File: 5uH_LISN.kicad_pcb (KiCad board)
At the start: 2 copper layers, 112.4 x 60.5 mm, 74 parts, among them J1 Conn_SMA, J2 Conn_SMA, J3 BANANA_CONN, J4 BANANA_CONN, J5 BANANA_CONN, J6 BANANA_CONN, J7 BANANA_CONN, J8 BANANA_CONN

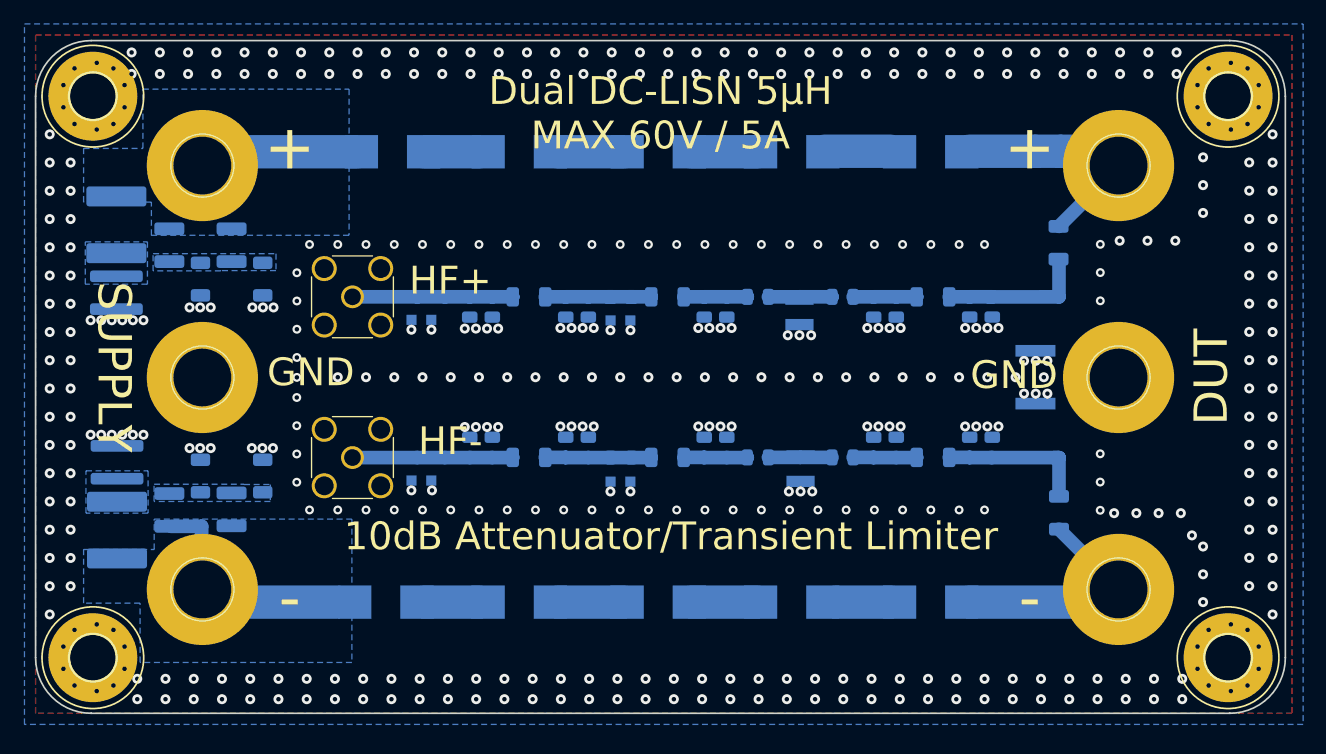
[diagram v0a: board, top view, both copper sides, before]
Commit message: redesign, see readme
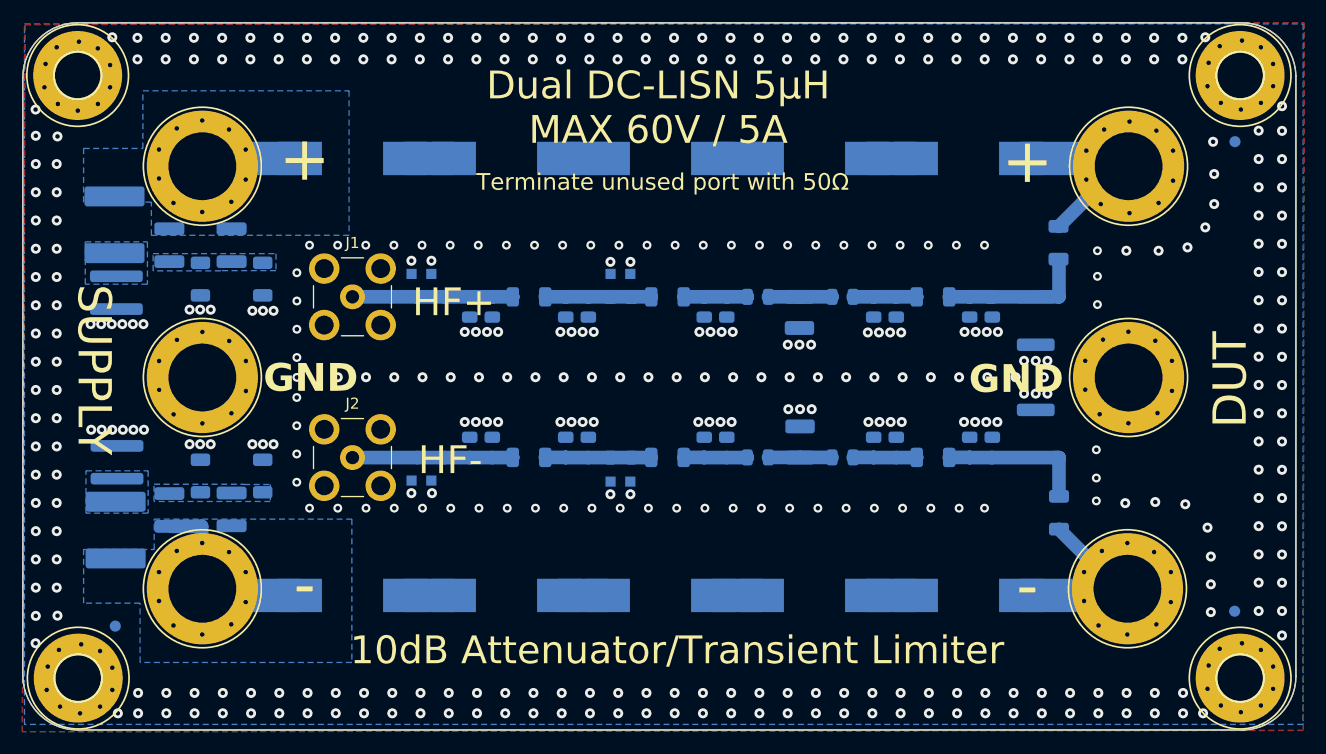
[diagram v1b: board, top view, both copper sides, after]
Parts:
- removed GD1, GD2: S30-A75X, 5uH_LISN:S30-A400X
- removed the L12 at (168.9, 118.5)
- removed the L6 at (168.8, 104.4)
- added CASE1: B013BK, 5uH_LISN:B013BK, F.Cu at (103.9, 83.1)
- added FID1: Fiducial, Fiducial:Fiducial_1mm_Mask2mm, B.Cu at (207.9, 89.1)
- added FID2: Fiducial, Fiducial:Fiducial_1mm_Mask2mm, B.Cu at (207.9, 131.3)
- added FID3: Fiducial, Fiducial:Fiducial_1mm_Mask2mm, B.Cu at (107.2, 132.6)
- added L7: 1mH, Inductor_SMD:L_1210_3225Metric, B.Cu at (168.8, 104.4)
- added L8: 1mH, Inductor_SMD:L_1210_3225Metric, B.Cu at (168.8, 116.1)
- added RF1: 132360, 5uH_LISN:RF_CAP, F.Cu at (128.6, 117.5)
- added U1: SMD75XM, Fuse:Fuse_1812_4532Metric, B.Cu at (190.0, 105.2)
- added U2: SMD75XM, Fuse:Fuse_1812_4532Metric, B.Cu at (190.0, 115.3)
- D1: renamed from D3; value SOT23-DIODEDUAL -> BAV99,215
- D2: renamed from D1; value SOT23-DIODEDUAL -> BAV99,215
- D3: renamed from D2; value SOT23-DIODEDUAL -> BAV99,215
- D4: value SOT23-DIODEDUAL -> BAV99,215
- J1, J2: footprint Connector_Coaxial:SMA_Wurth_60312002114503_Vertical -> Connector_Coaxial:SMB_Jack_Vertical
- J3, J4, J5, J6, J7, J8: footprint 5uH_LISN:BANANA_CONN -> 5uH_LISN:6,1-PAD
- L1: renamed from L7; value 1.1uH -> 1.0uH; footprint 5uH_LISN:WE-HCI_7030_7040_7050 -> 5uH_LISN:SMS1040
- L10: value 1.1uH -> 1.0uH; footprint 5uH_LISN:WE-HCI_7030_7040_7050 -> 5uH_LISN:SMS1040
- L11: renamed from L5; value 1.1uH -> 1.0uH; footprint 5uH_LISN:WE-HCI_7030_7040_7050 -> 5uH_LISN:SMS1040
- L12: renamed from L11; value 1.1uH -> 1.0uH; footprint 5uH_LISN:WE-HCI_7030_7040_7050 -> 5uH_LISN:SMS1040
- L2: renamed from L1; value 1.1uH -> 1.0uH; footprint 5uH_LISN:WE-HCI_7030_7040_7050 -> 5uH_LISN:SMS1040
- L3: renamed from L2; value 1.1uH -> 1.0uH; footprint 5uH_LISN:WE-HCI_7030_7040_7050 -> 5uH_LISN:SMS1040
- L4: renamed from L8; value 1.1uH -> 1.0uH; footprint 5uH_LISN:WE-HCI_7030_7040_7050 -> 5uH_LISN:SMS1040
- L5: renamed from L3; value 1.1uH -> 1.0uH; footprint 5uH_LISN:WE-HCI_7030_7040_7050 -> 5uH_LISN:SMS1040
- L6: renamed from L9; value 1.1uH -> 1.0uH; footprint 5uH_LISN:WE-HCI_7030_7040_7050 -> 5uH_LISN:SMS1040
- L9: renamed from L4; value 1.1uH -> 1.0uH; footprint 5uH_LISN:WE-HCI_7030_7040_7050 -> 5uH_LISN:SMS1040
- moved J7 38.1 mm to (198.3, 129.3)
- moved J5 38.1 mm to (115.1, 91.3)
- moved J8 19.1 mm to (198.4, 110.3)
- moved J3 19.1 mm to (115.1, 110.3)
- moved J6 19.0 mm to (198.4, 91.3)
- moved J4 19.0 mm to (115.1, 129.3)
- moved L2 3.65 mm to (128.6, 90.6)
- moved L11 3.45 mm to (184.0, 90.6)
- moved L12 3.45 mm to (184.0, 129.9)
- moved L1 3.06 mm to (128.6, 129.9)
- moved H2 2.31 mm to (103.9, 83.1)
- moved H1 2.26 mm to (103.9, 137.3)
- moved H3 2.16 mm to (208.4, 83.1)
- moved D3 2.15 mm to (152.7, 102.0), turned to 180 degrees
- moved L10 2.14 mm to (170.1, 129.9)
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- renumbered C14 to C10, C15 to C11, C16 to C12, C5 to C3, C6 to C4, C7 to C5, C8 to C6, C11 to C7, C12 to C8, C13 to C9
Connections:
- C1 pad 1: Net-(C1-Pad1) -> Net-(J5-P)
- C11 pad 1: Net-(C15-Pad1) -> Net-(J6-P)
- C12 pad 1: Net-(C16-Pad1) -> Net-(J7-P)
- C2 pad 1: Net-(C2-Pad1) -> Net-(J4-P)
- C3 pad 1: Net-(C1-Pad1) -> Net-(J5-P)
- C4 pad 1: Net-(C2-Pad1) -> Net-(J4-P)
- C5 pad 1: Net-(C1-Pad1) -> Net-(J5-P)
- C6 pad 1: Net-(C2-Pad1) -> Net-(J4-P)
- L1 pad 1: Net-(C2-Pad1) -> Net-(J4-P)
- L11 pad 2: Net-(C15-Pad1) -> Net-(J6-P)
- L12 pad 2: Net-(C16-Pad1) -> Net-(J7-P)
- L2 pad 1: Net-(C1-Pad1) -> Net-(J5-P)
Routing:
- net Net-(C15-Pad1): track 22.4 -> 0.00 mm
- net Net-(C16-Pad1): track 22.3 -> 0.00 mm
- net Net-(C2-Pad1): track 21.7 -> 0.00 mm
- net Net-(J4-P): track 0.00 -> 18.6 mm, vias 0 -> 10
- net Net-(J6-P): track 0.00 -> 18.0 mm, vias 0 -> 10
- net Net-(J7-P): track 0.00 -> 17.8 mm, vias 0 -> 10
- net Net-(C1-Pad1): track 13.9 -> 0.00 mm
- net Net-(J5-P): track 0.00 -> 9.02 mm, vias 0 -> 10
- net Net-(L10-Pad2): track 9.30 -> 4.35 mm
- net Net-(L5-Pad2): track 6.00 -> 4.35 mm
- net Net-(L11-Pad1): track 6.00 -> 4.35 mm
- net Net-(L10-Pad1): track 6.00 -> 4.35 mm
- net Net-(L4-Pad2): track 6.00 -> 4.35 mm
- net Net-(L3-Pad2): track 6.00 -> 4.35 mm
- net Net-(L2-Pad2): track 5.00 -> 4.35 mm
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- added copper zone on B.Cu, net Net-(J4-P)
- added copper zone on B.Cu, net Net-(J5-P)
- removed copper zone on B.Cu, net Net-(C1-Pad1)
- removed copper zone on B.Cu, net Net-(C2-Pad1)
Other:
- board size 112.4 x 60.5 mm -> 114.5 x 63.6 mm
- board text added: "Dual DC-LISN 5µH board spec.: X: 114.5 mm Y: 63.6 mm 2 conductive layers, FR4, 1,60 mm. First Top Layer: F.Cu, foil 0.035 mm; Second Bottom Layer: B.Cu, foil 0.035 mm Surface Finish: HASL Lead Free TOP: Mask - Black, Mark - White BOTTOM: Mask - Black, Mark - White Contacts: POS-63 Holes diameter size not less 0.4 mm Min conductor width on outer/inner layers 0.63 mm"
- board text added: "Terminate unused port with 50Ω"
- board text added: "V1 R1 25.04.2024"
- board text removed: "V1 R0 12Dec2021"
